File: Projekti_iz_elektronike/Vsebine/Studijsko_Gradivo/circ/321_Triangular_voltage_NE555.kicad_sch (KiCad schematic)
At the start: 8 parts, among them Q1 PNP, U1 NE555P

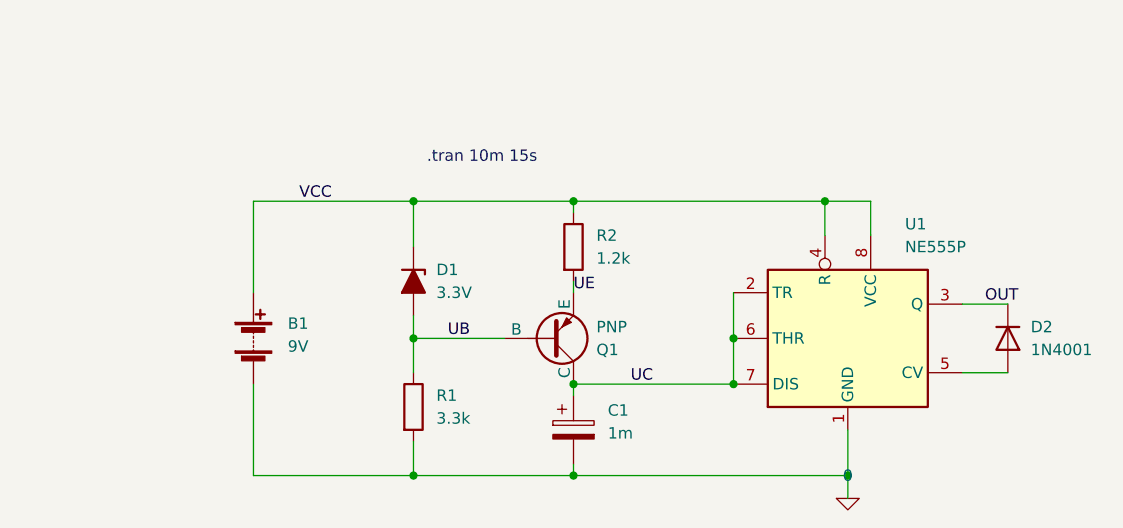
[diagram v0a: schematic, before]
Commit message: gradivo
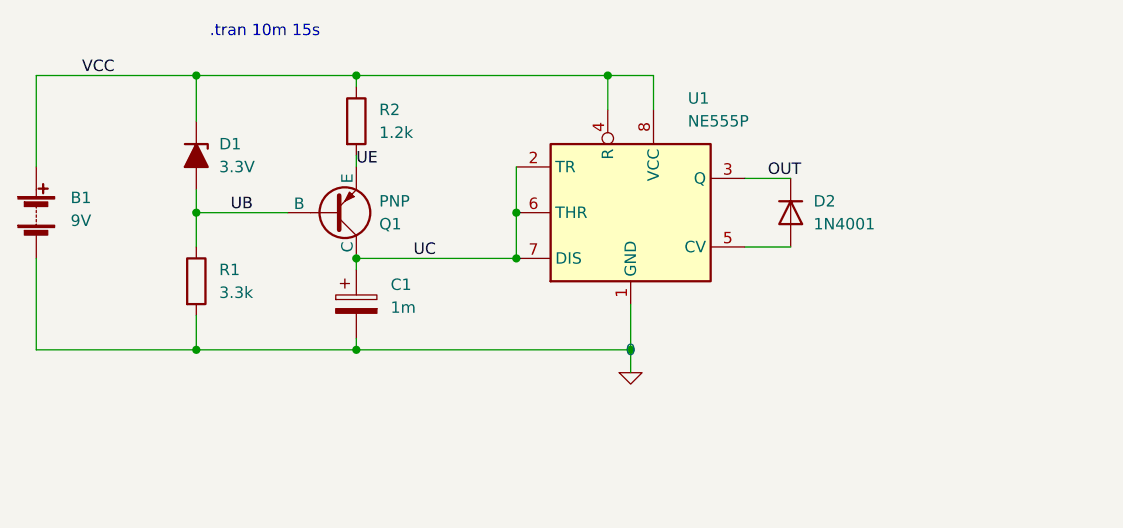
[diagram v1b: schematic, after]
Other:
- moved on the sheet: B1, C1, D1, D2, Q1, R1, R2, U1
